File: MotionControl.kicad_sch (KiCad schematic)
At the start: 22 parts, among them J2 Conn_ARM_JTAG_SWD_10, Q1 2N7002, SW1 SW_Push, U1 ATSAMD21J18A-A, Y1 32.768kHz

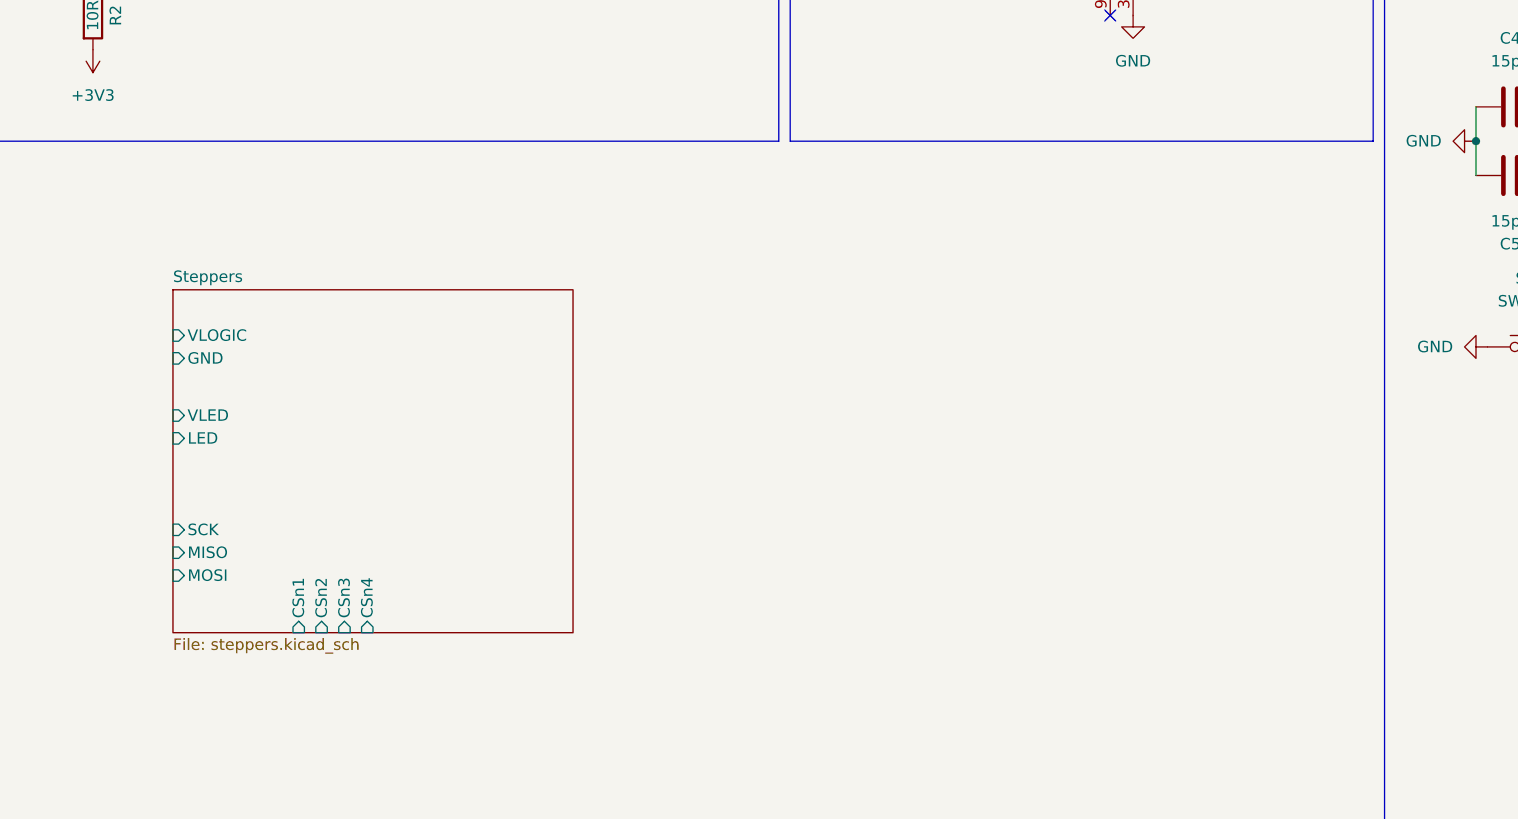
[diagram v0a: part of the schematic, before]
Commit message: Lots of work
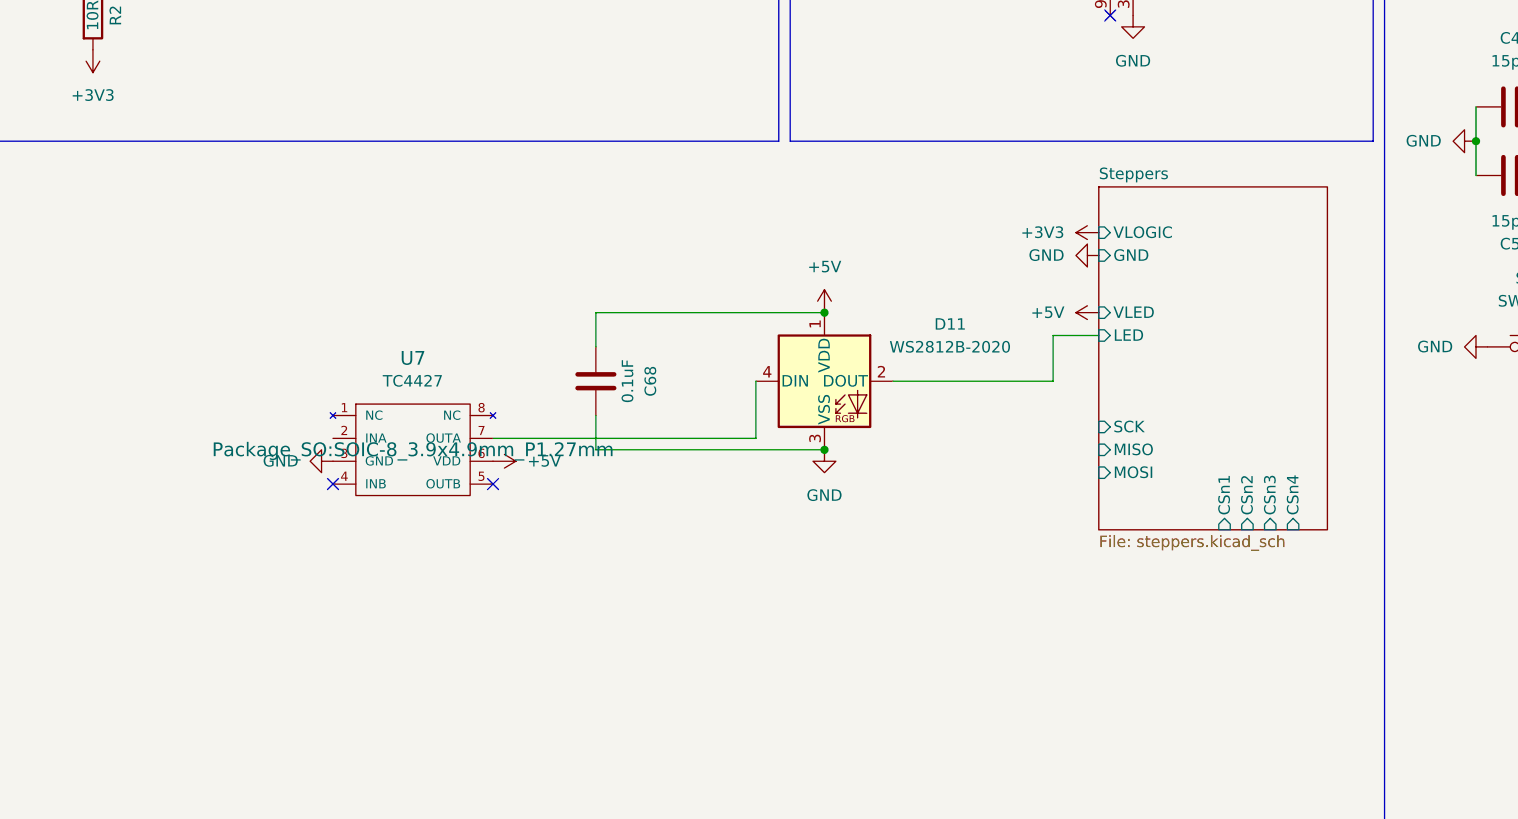
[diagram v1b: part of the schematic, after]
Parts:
- added C68: 0.1uF, Capacitor_SMD:C_0402_1005Metric, symbol Device:C
- added D11: WS2812B-2020, LED_SMD:LED_WS2812B-Mini_PLCC4_3.5x3.5mm, symbol LED:WS2812B
- added U7: TC4427, Package_SO:SOIC-8_3.9x4.9mm_P1.27mm, symbol Driver_FET2:TC4427
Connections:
- net +5V: now also C68.1, D11.1 (VDD), U7.6 (VDD)
- net GND: now also C68.2, D11.3 (VSS), U7.3 (GND)
- net Steppers/LED: now also D11.2 (DOUT)
- new net: D11.4 (DIN), U7.7 (OUTA)
- no-connect marks 3 -> 5
